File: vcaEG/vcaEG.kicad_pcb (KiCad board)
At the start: 2 copper layers, 37 parts, among them J1 Conn_01x10_MountingPin, Q1 BC307, Q2 BC237, Q3 BC237, Q4 BC237, Q5 BC237, SW1 SW_Rotary2x3, U1 TL071

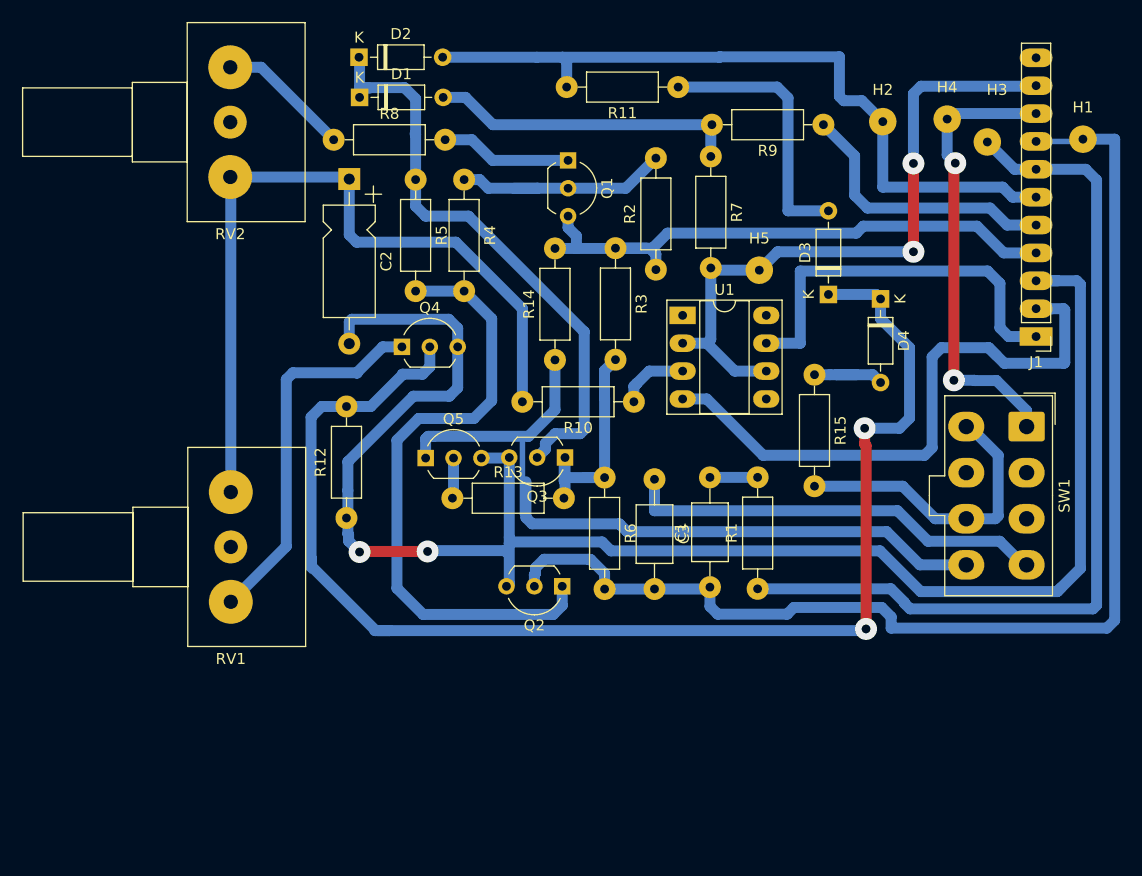
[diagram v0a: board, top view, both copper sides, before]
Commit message: Add files via upload
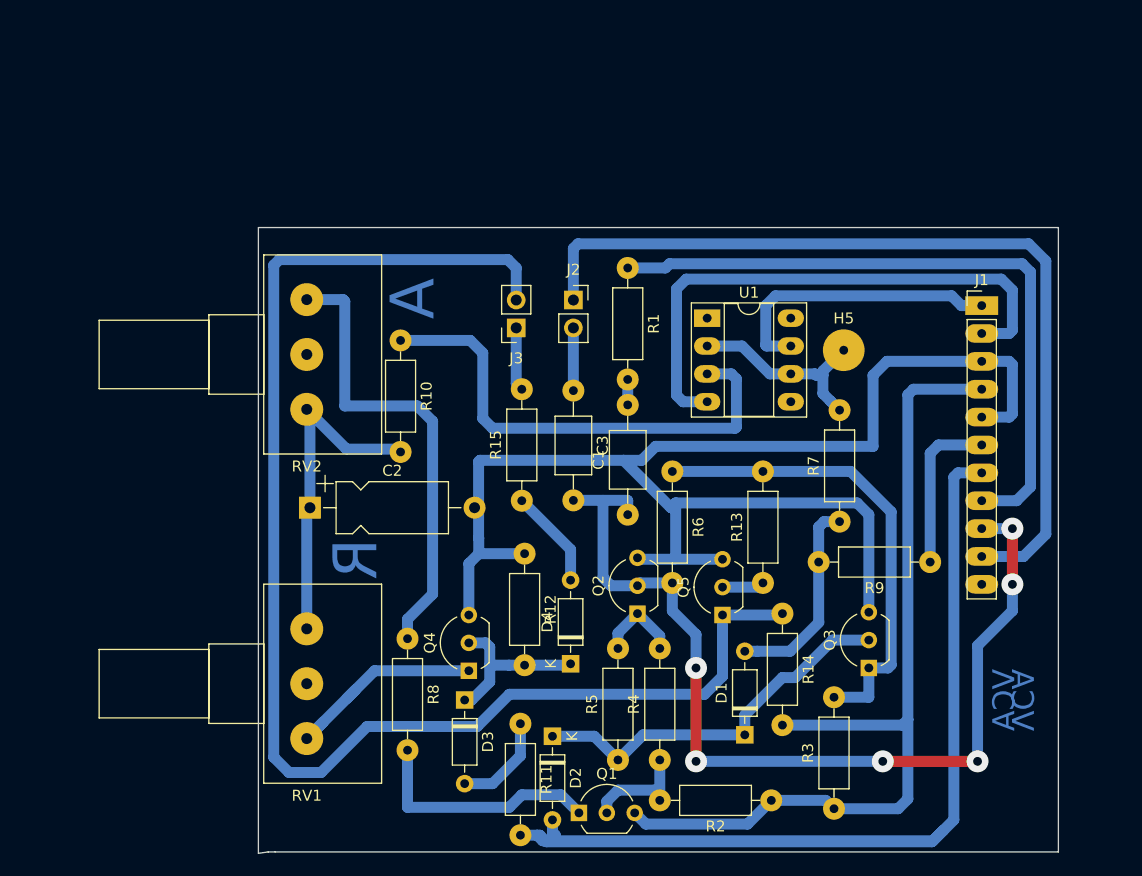
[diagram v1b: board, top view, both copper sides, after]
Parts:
- removed H1, H2, H3, H4: MountingHole_Pad, MountingHole:MountingHole_2.2mm_M2_DIN965_Pad
- removed SW1: SW_Rotary2x3, Connector_Molex:Molex_Mini-Fit_Jr_5566-08A_2x04_P4.20mm_Vertical
- added J2: Conn_01x02_MountingPin, Connector_PinSocket_2.54mm:PinSocket_1x02_P2.54mm_Vertical, F.Cu at (74.3, 50.0)
- added J3: Conn_01x02_MountingPin, Connector_PinSocket_2.54mm:PinSocket_1x02_P2.54mm_Vertical, F.Cu at (69.1, 52.6)
- moved D1 67.9 mm to (89.9, 89.7), turned to 90 degrees
- moved D2 64.3 mm to (72.4, 89.8), turned to 270 degrees
- moved R11 59.8 mm to (69.5, 88.6), turned to 270 degrees
- moved Q1 59.5 mm to (74.8, 96.8), turned to 0 degrees
- moved R5 56.0 mm to (78.4, 91.9), turned to 90 degrees
- moved R4 55.8 mm to (82.2, 91.9), turned to 90 degrees
- moved R3 54.8 mm to (98.0, 96.4), turned to 90 degrees
- moved D3 49.6 mm to (64.4, 86.5), turned to 270 degrees
- moved R2 49.5 mm to (92.3, 95.6), turned to 180 degrees
- moved R8 46.0 mm to (59.2, 80.9), turned to 270 degrees
- moved D4 43.6 mm to (74.0, 83.2), turned to 90 degrees
- moved R9 41.0 mm to (106.8, 73.9)
- moved R7 35.3 mm to (98.6, 70.2), turned to 90 degrees
- moved Q3 33.7 mm to (101.2, 83.6), turned to 90 degrees
- moved R1 31.5 mm to (79.2, 47.1), turned to 270 degrees
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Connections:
- J1 pad 10: Net-(H5-Pad1) -> Net-(J1-Pad10)
- J1 pad 5: -8V -> GND
- J1 pad 6: Net-(D2-Pad2) -> -8V
- J1 pad 7: Net-(H3-Pad1) -> Net-(D2-Pad2)
- J1 pad 8: Net-(C1-Pad1) -> Net-(J1-Pad8)
- J1 pad 9: Net-(H4-Pad1) -> Net-(C1-Pad1)
- R1 pad 1: Net-(H3-Pad1) -> Net-(J1-Pad8)
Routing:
- net Net-(D3-Pad1): track 122.7 -> 15.6 mm, vias 2 -> 0
- net Net-(H3-Pad1): track 82.0 -> 0.00 mm
- net Net-(J1-Pad10): track 0.00 -> 80.2 mm
- net Net-(J1-Pad8): track 0.00 -> 62.8 mm
- net Net-(Q2-Pad1): track 57.2 -> 7.93 mm
- net Net-(D2-Pad2): track 67.9 -> 114.1 mm
- net Net-(H5-Pad1): track 60.8 -> 18.5 mm, vias 2 -> 0
- net Net-(H4-Pad1): track 41.7 -> 0.00 mm, vias 2 -> 0
- net Net-(C2-Pad1): track 71.8 -> 30.5 mm
- net Net-(R10-Pad1): track 6.43 -> 44.7 mm
- net Net-(J3-Pad2): track 89.0 -> 126.6 mm
- net Net-(C3-Pad1): track 38.8 -> 5.71 mm
- net Net-(R8-Pad1): track 12.2 -> 42.4 mm
- net +7.5V: track 54.8 -> 82.3 mm
- net GND: track 154.5 -> 128.9 mm, vias 2 -> 0
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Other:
- board outline added: 72.9 x 57 mm
- net class Default: clearance 0.2 -> 0.4
- rule trace_clearance: 0.2 -> 0.4
- board text added: "A"
- board text added: "R"
- board text added: "VCA"
